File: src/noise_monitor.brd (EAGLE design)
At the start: 53 x 48 mm, 72 parts, among them IC2 MCP73831/OT, T1 S8050, T2 S8050, U2 TEXAS_INSTRUMENTS_SN74HC125TE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, U4 ESP8266-12E/ESP-12E, U5 CP2102N-A02-GQFN28, U6 LP2989AILD-3.3, X2 SIMLOCK-C707_10M006_512_2

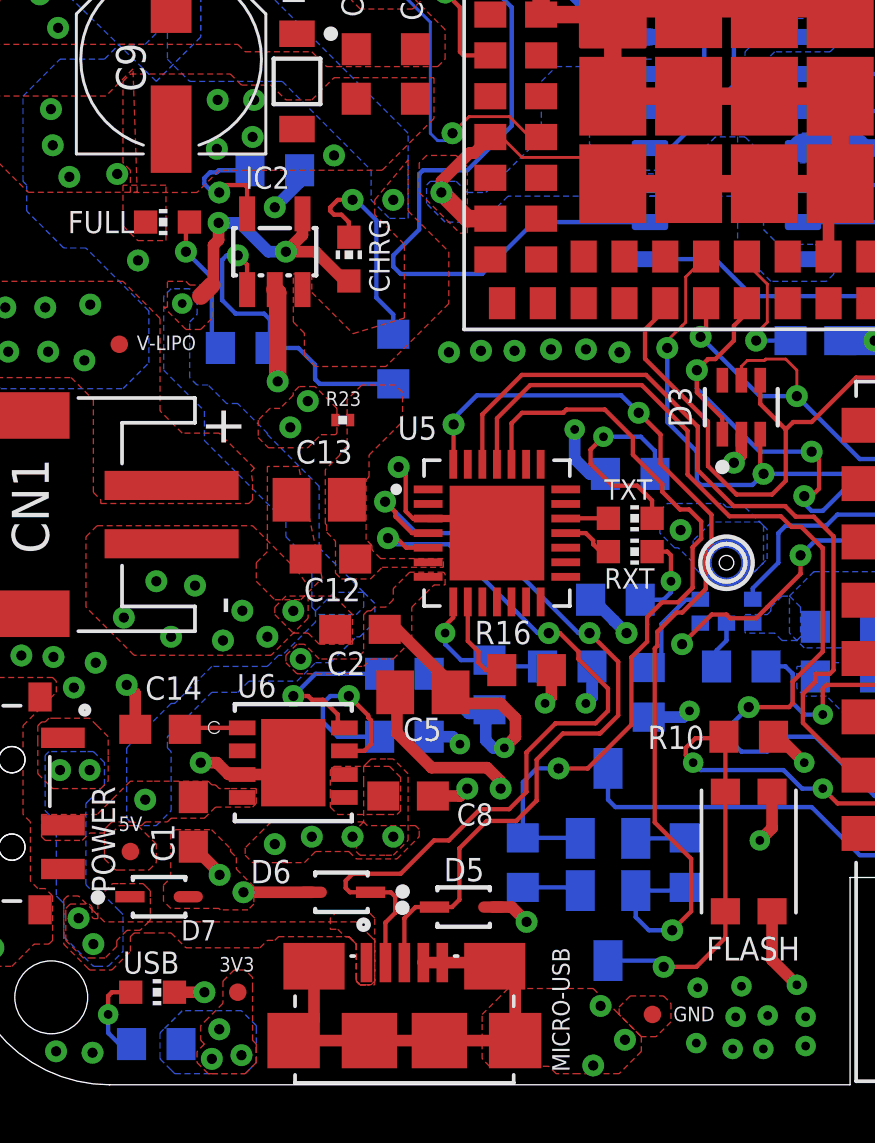
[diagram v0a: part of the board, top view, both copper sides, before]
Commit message: Added CAM files
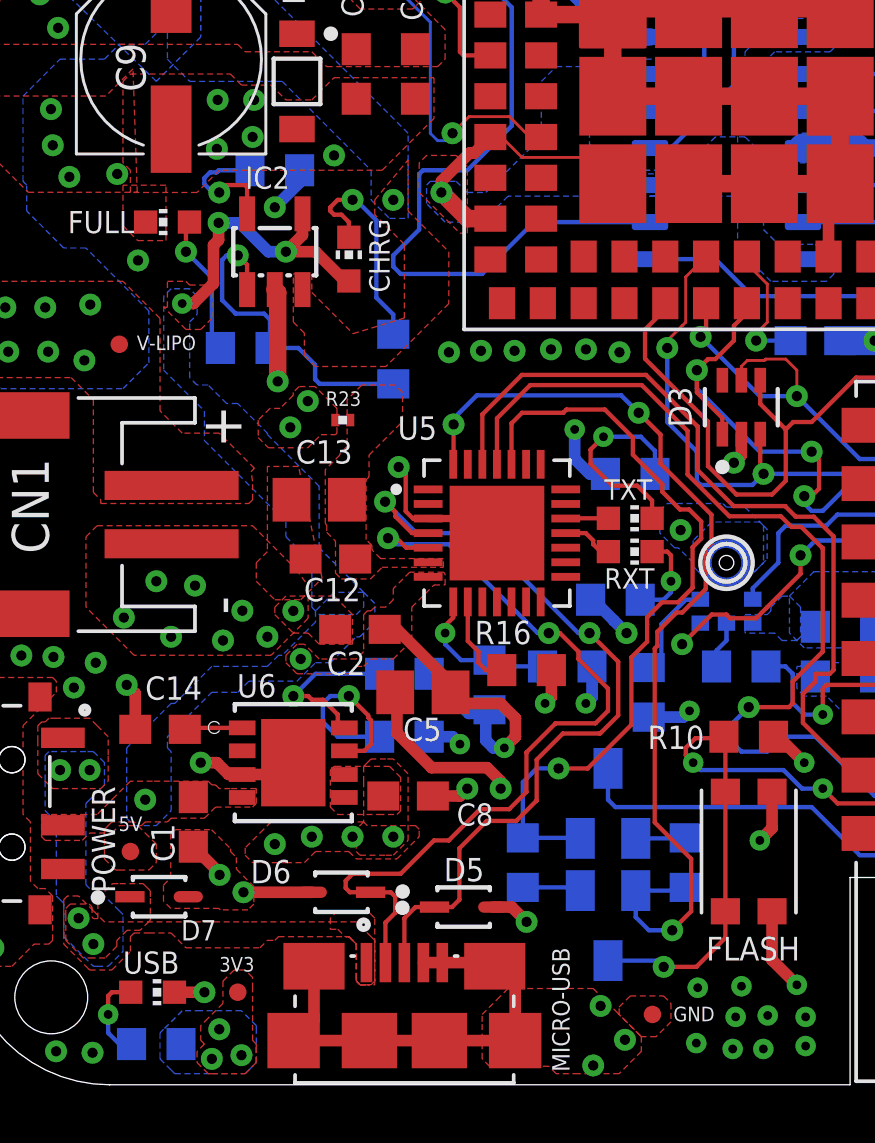
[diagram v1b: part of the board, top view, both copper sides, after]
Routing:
- net GND: track 142.5 -> 139.8 mm
- net +5V: track 21.4 -> 21.9 mm
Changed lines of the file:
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@@
 <drawing>
 <settings>
-<setting alwaysvectorfont="yes"/>
+<setting alwaysvectorfont="no"/>
 <setting verticaltext="up"/>
 </settings>
@@
 <wire x1="32.779365625" y1="22.596228125" x2="33.147" y2="22.206" width="0.8" layer="1"/>
 <via x="33.147" y="22.206" extent="1-16" drill="0.35"/>
-<wire x1="15.763" y1="4.191" x2="15.748" y2="4.206" width="0.4" layer="1"/>
 <wire x1="16.413" y1="4.191" x2="18.088" y2="4.191" width="0.4" layer="1"/>
 <wire x1="18.088" y1="4.191" x2="18.213" y2="4.066" width="0.4" layer="1"/>
-<wire x1="22.262" y1="30.909" x2="24.844" y2="30.909" width="0.6" layer="1"/>
-<wire x1="24.844" y1="30.909" x2="24.892" y2="30.861" width="0.6" layer="1"/>
 <wire x1="27.462" y1="30.909" x2="24.862" y2="30.909" width="0.6" layer="1"/>
 <wire x1="27.462" y1="30.909" x2="29.718" y2="30.909" width="0.6" layer="1"/>
@@
 <wire x1="9.0863125" y1="10.6426" x2="8.6799125" y2="11.049" width="0.4" layer="1"/>
 <via x="8.128" y="11.049" extent="1-16" drill="0.35"/>
-<wire x1="9.5504" y1="10.6426" x2="9.5758" y2="10.668" width="0.4" layer="1"/>
 <via x="14.917" y="21.19" extent="1-16" drill="0.35"/>
 <wire x1="16.09" y1="9.906" x2="17.018" y2="9.906" width="0.4" layer="1"/>
@@
 <contactref element="IC2" pad="4"/>
 <contactref element="CHRG" pad="A"/>
-<wire x1="8.128" y1="27.051" x2="8.509" y2="27.432" width="0.6" layer="1"/>
-<wire x1="8.509" y1="27.432" x2="8.5658" y2="27.4888" width="0.4" layer="1"/>
 <wire x1="8.74" y1="28.9763125" x2="8.5658" y2="28.8021125" width="0.4" layer="1"/>
 <wire x1="8.74" y1="28.9763125" x2="8.74" y2="29.564" width="0.4" layer="1"/>
-<wire x1="8.5658" y1="27.4888" x2="8.5658" y2="28.8021125" width="0.4" layer="1"/>
+<wire x1="8.5658" y1="28.8021125" x2="8.5658" y2="27.4888" width="0.4" layer="1"/>
 <via x="8.74" y="29.564" extent="1-16" drill="0.35"/>
 <wire x1="8.74" y1="29.564" x2="9.4589125" y2="29.564" width="0.4" layer="16"/>
@@
 <via x="11.557" y="14.605" extent="1-16" drill="0.35"/>
 <wire x1="14.3546875" y1="15.621" x2="14.439" y2="15.621" width="0.4" layer="1"/>
-<wire x1="14.439" y1="15.621" x2="14.605" y2="15.787" width="0.4" layer="1"/>
 <polygon width="0.1" layer="16">
 <vertex x="11.938" y="16.383"/>
@@
 <wire x1="15.963" y1="14.097" x2="17.321" y2="12.739" width="0.4" layer="16"/>
 <wire x1="17.321" y1="12.739" x2="17.907" y2="12.739" width="0.4" layer="16"/>
+<wire x1="7.874" y1="26.797" x2="7.493" y2="26.797" width="0.4" layer="1"/>
+<wire x1="8.5658" y1="27.4888" x2="7.874" y2="26.797" width="0.4" layer="1"/>
 </signal>
 <signal name="+3V3" class="1">
